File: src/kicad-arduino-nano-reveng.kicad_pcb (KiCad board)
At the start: 2 copper layers, 43.8 x 18.4 mm, 14 parts

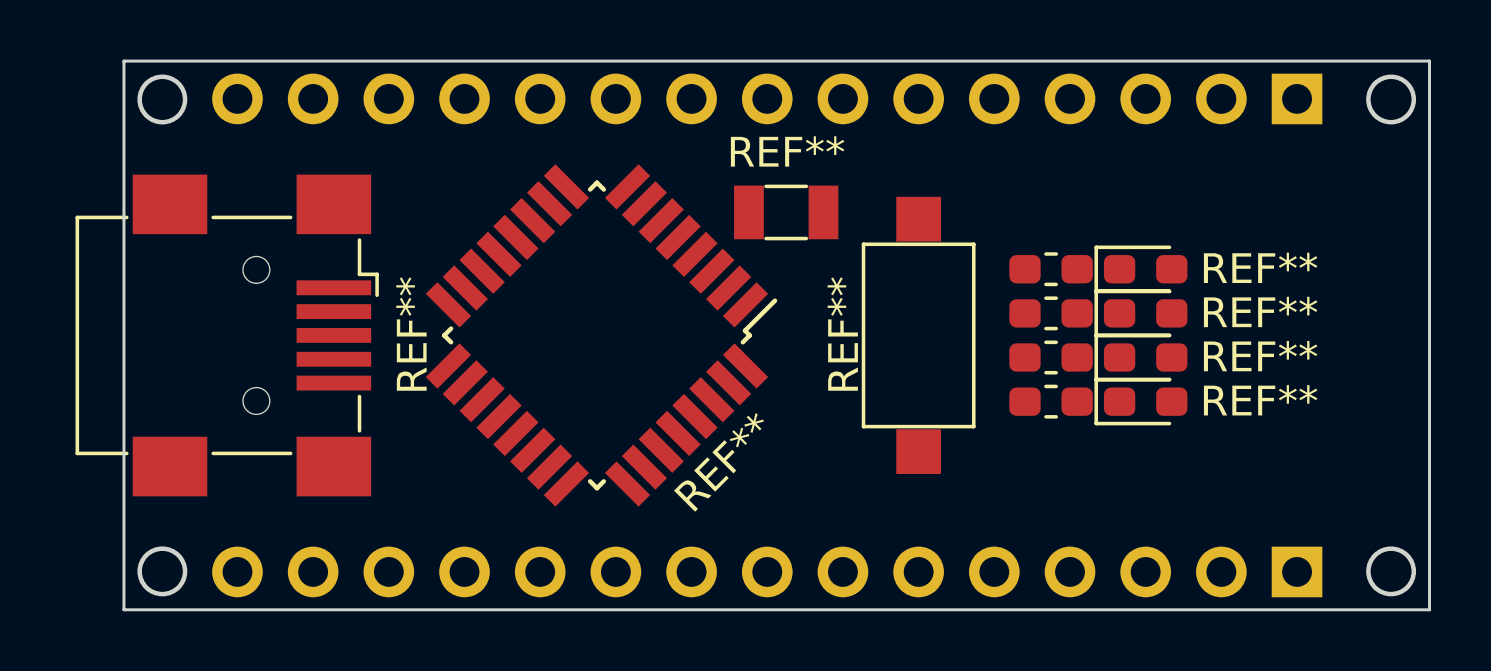
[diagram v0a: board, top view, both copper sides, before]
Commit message: back layer components
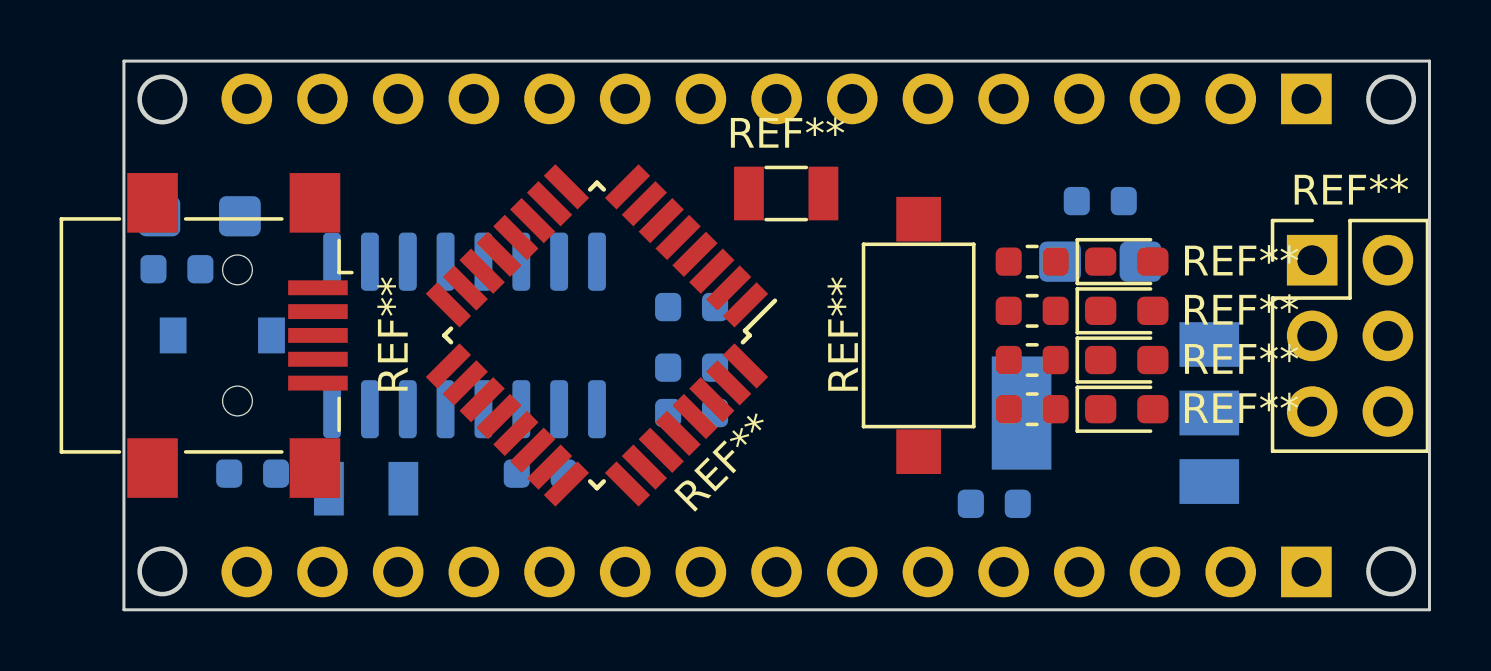
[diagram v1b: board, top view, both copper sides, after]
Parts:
- removed the REF** at (111.8, 59.1)
- removed the REF** at (111.8, 57.6)
- removed the REF** at (111.8, 56.1)
- added REF**: Crystal_SMD_MicroCrystal_CC7V-T1A-2Pin_3.2x1.5mm, Crystal:Crystal_SMD_MicroCrystal_CC7V-T1A-2Pin_3.2x1.5mm, B.Cu at (85.6, 62.0)
- added REF**: C_0603_1608Metric, Capacitor_SMD:C_0603_1608Metric, B.Cu at (81.8, 61.5)
- added REF**: C_0603_1608Metric, Capacitor_SMD:C_0603_1608Metric, B.Cu at (91.4, 61.5)
- added REF**: C_0603_1608Metric, Capacitor_SMD:C_0603_1608Metric, B.Cu at (96.5, 55.9)
- added REF**: SOT-223, Package_TO_SOT_SMD:SOT-223, B.Cu at (110.7, 59.4)
- added REF**: SOIC-16_3.9x9.9mm_P1.27mm, Package_SO:SOIC-16_3.9x9.9mm_P1.27mm, B.Cu at (88.9, 56.8)
- added REF**: PinHeader_2x03_P2.54mm_Vertical, Connector_PinHeader_2.54mm:PinHeader_2x03_P2.54mm_Vertical, F.Cu at (117.3, 54.3)
- added REF**: C_0603_1608Metric, Capacitor_SMD:C_0603_1608Metric, B.Cu at (110.2, 52.3)
- added REF**: LED_0603_1608Metric_Pad1.05x0.95mm_HandSolder, LED_SMD:LED_0603_1608Metric_Pad1.05x0.95mm_HandSolder, F.Cu at (111.1, 59.3)
- added REF**: LED_0603_1608Metric_Pad1.05x0.95mm_HandSolder, LED_SMD:LED_0603_1608Metric_Pad1.05x0.95mm_HandSolder, F.Cu at (111.1, 57.7)
- added REF**: LED_0603_1608Metric_Pad1.05x0.95mm_HandSolder, LED_SMD:LED_0603_1608Metric_Pad1.05x0.95mm_HandSolder, F.Cu at (111.1, 56.0)
- added REF**: CP_EIA-3216-10_Kemet-I, Capacitor_Tantalum_SMD:CP_EIA-3216-10_Kemet-I, B.Cu at (110.2, 54.4)
- added REF**: CP_EIA-3216-10_Kemet-I, Capacitor_Tantalum_SMD:CP_EIA-3216-10_Kemet-I, B.Cu at (80.0, 52.8)
- added REF**: C_0603_1608Metric, Capacitor_SMD:C_0603_1608Metric, B.Cu at (79.2, 54.6)
- added REF**: D_SOD-123, Diode_SMD:D_SOD-123, B.Cu at (80.8, 56.8)
- added REF**: R_0603_1608Metric, Resistor_SMD:R_0603_1608Metric, B.Cu at (96.5, 57.9)
- added REF**: R_0603_1608Metric, Resistor_SMD:R_0603_1608Metric, B.Cu at (96.5, 59.4)
- added e: R_0603_1608Metric, Resistor_SMD:R_0603_1608Metric, B.Cu at (106.7, 62.5)
- REF** (x4): value R_0603_1608Metric_Pad1.05x0.95mm_HandSolder -> R_0603_1608Metric; footprint Resistor_SMD:R_0603_1608Metric_Pad1.05x0.95mm_HandSolder -> Resistor_SMD:R_0603_1608Metric
- REF**: value USB_Mini-B_Wuerth_65100516121_Horizontal -> USB_Mini-B_Lumberg_2486_01_Horizontal; footprint Connector_USB:USB_Mini-B_Wuerth_65100516121_Horizontal -> Connector_USB:USB_Mini-B_Lumberg_2486_01_Horizontal
- moved REF** 0.68 mm to (111.1, 54.4)
- moved REF** 0.68 mm to (108.0, 59.3)
- moved REF** 0.68 mm to (108.0, 54.4)
- moved REF** 0.64 mm to (108.0, 56.0)
- moved REF** 0.64 mm to (108.0, 57.7)
- moved REF** 0.64 mm to (81.3, 56.8)
- moved REF** 0.63 mm to (99.7, 52.1)
- moved REF** 0.31 mm to (117.2, 48.9)
- moved REF** 0.31 mm to (117.2, 64.8)
